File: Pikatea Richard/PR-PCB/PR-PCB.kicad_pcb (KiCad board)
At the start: 2 copper layers, 62 x 136.7 mm, 7 parts, among them SW1 Rotary_Encoder_Switch, SW2 Rotary_Encoder_Switch

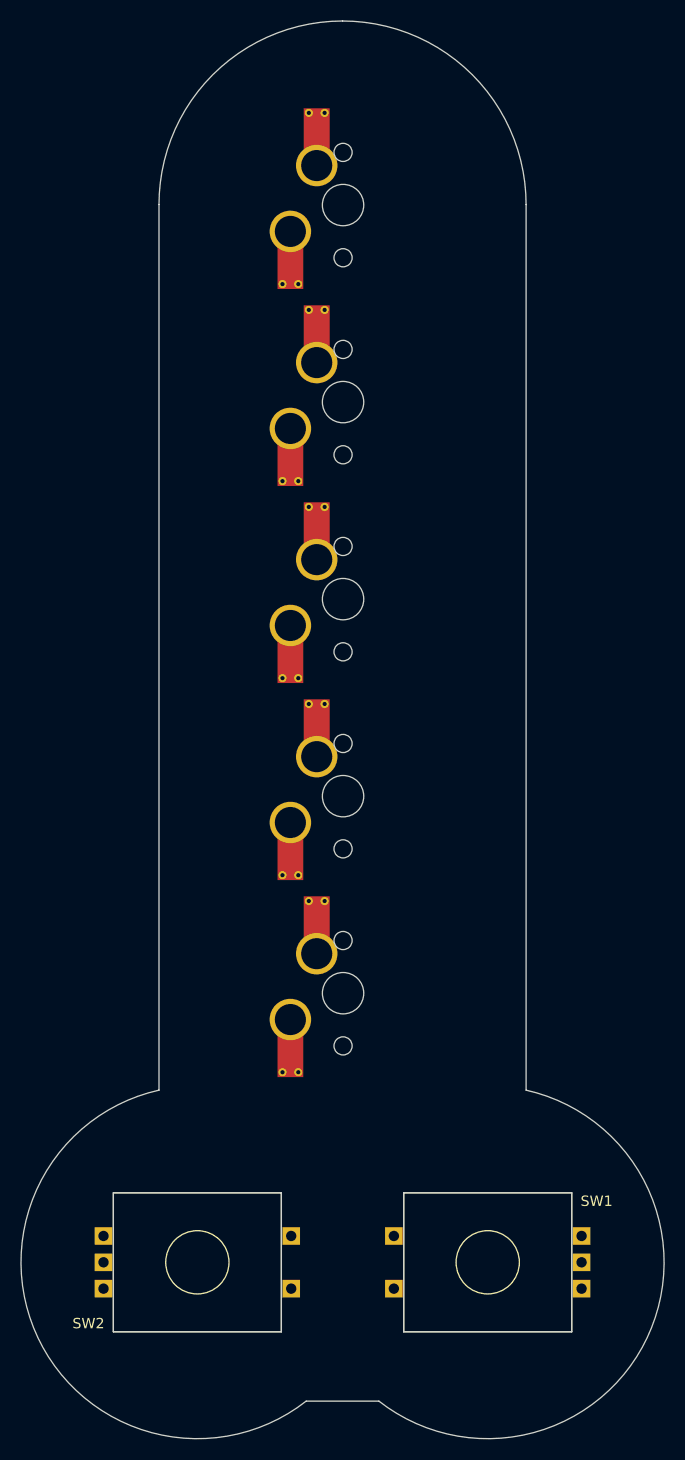
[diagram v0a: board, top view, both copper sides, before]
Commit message: updated footprints added gerbers
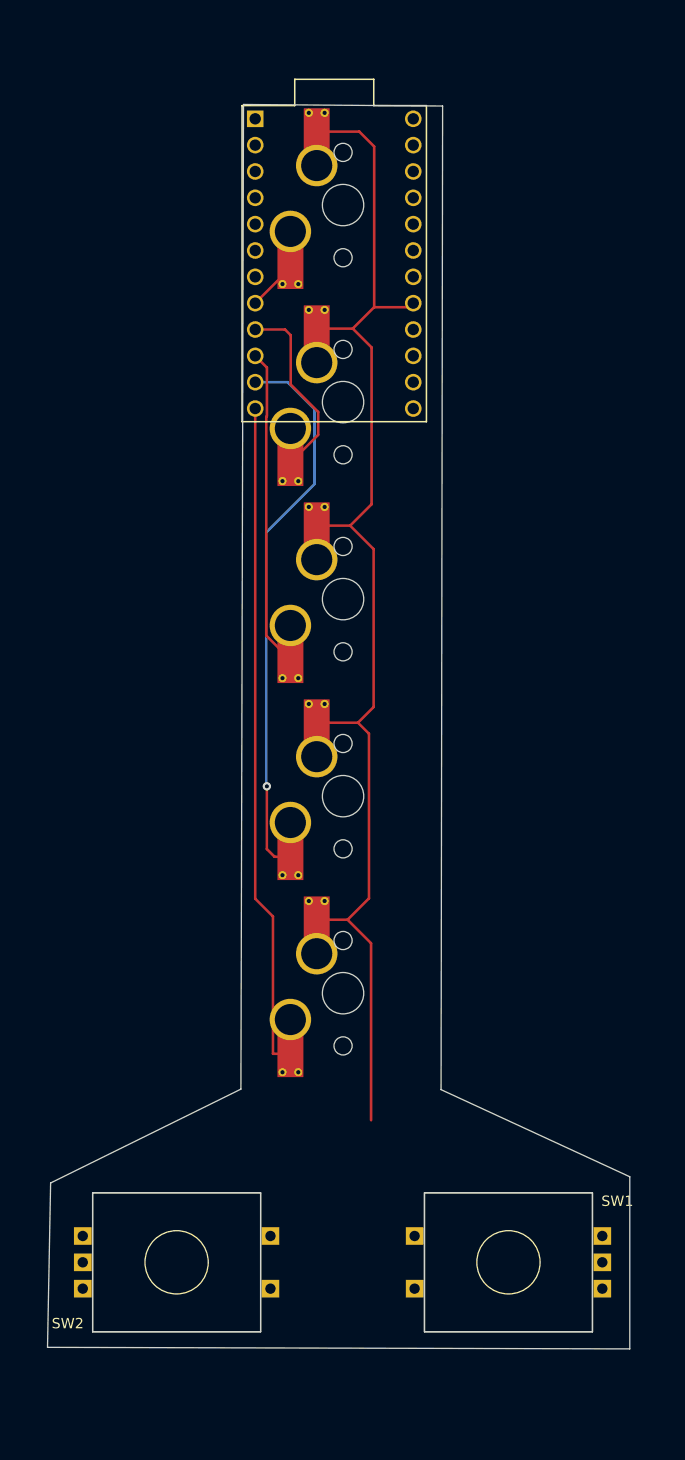
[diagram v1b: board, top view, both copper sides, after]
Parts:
- added U1: ProMicro, promicro:ProMicro, F.Cu at (138.2, 3.70)
- moved SW1 2.00 mm to (155.0, 100.0)
- moved SW2 2.00 mm to (123.0, 100.0)
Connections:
- MX2 pad 1: Net-(MX2-Pad1) -> Net-(MX1-Pad1)
- MX3 pad 1: Net-(MX3-Pad1) -> Net-(MX1-Pad1)
- MX4 pad 1: Net-(MX4-Pad1) -> Net-(MX1-Pad1)
- MX5 pad 1: Net-(MX5-Pad1) -> Net-(MX1-Pad1)
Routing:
- net Net-(MX1-Pad1): track 0.00 -> 123.9 mm
- net Net-(MX1-Pad2): track 0.00 -> 64.6 mm
- net Net-(MX2-Pad2): track 0.00 -> 53.7 mm, vias 0 -> 1
- net Net-(MX3-Pad2): track 0.00 -> 30.8 mm
- net Net-(MX4-Pad2): track 0.00 -> 18.1 mm
- net Net-(MX5-Pad2): track 0.00 -> 5.02 mm
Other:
- board size 62 x 136.7 mm -> 56.1 x 120 mm
